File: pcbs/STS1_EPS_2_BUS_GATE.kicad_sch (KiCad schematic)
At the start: 19 parts, among them Q5 SI7135DP-T1-GE3, Q6 2N7002, U13 4082, U3 TPS2420RSAT

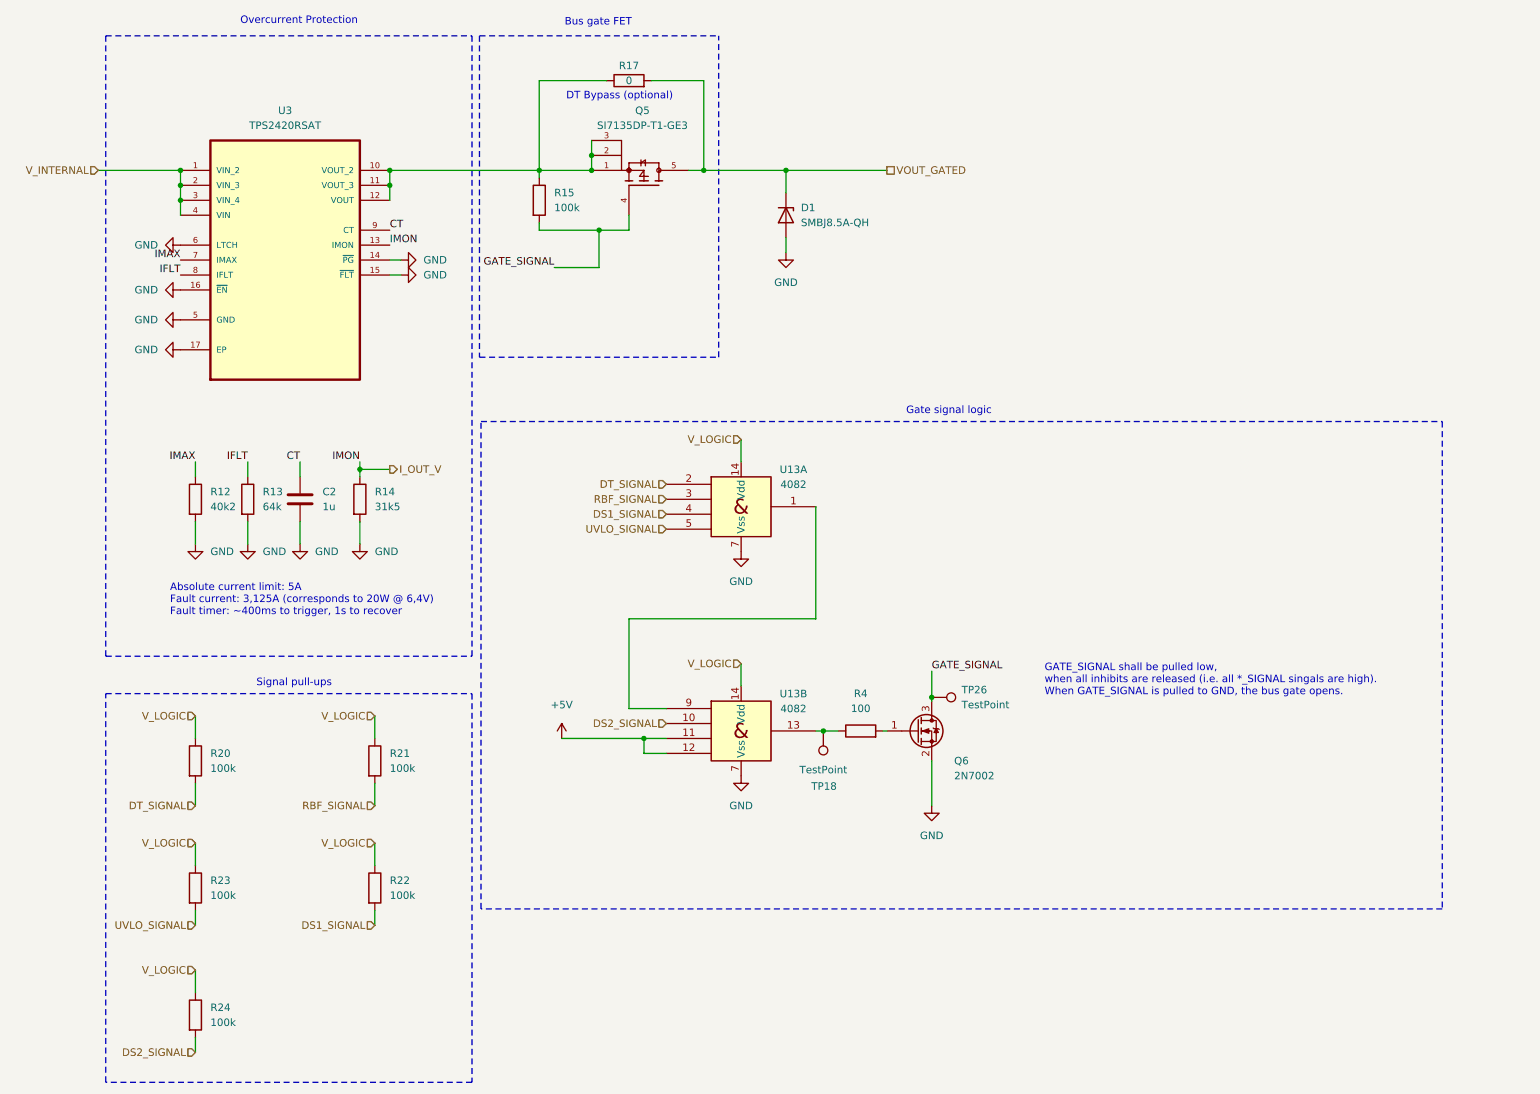
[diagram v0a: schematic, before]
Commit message: Fixed some warnings and errors.
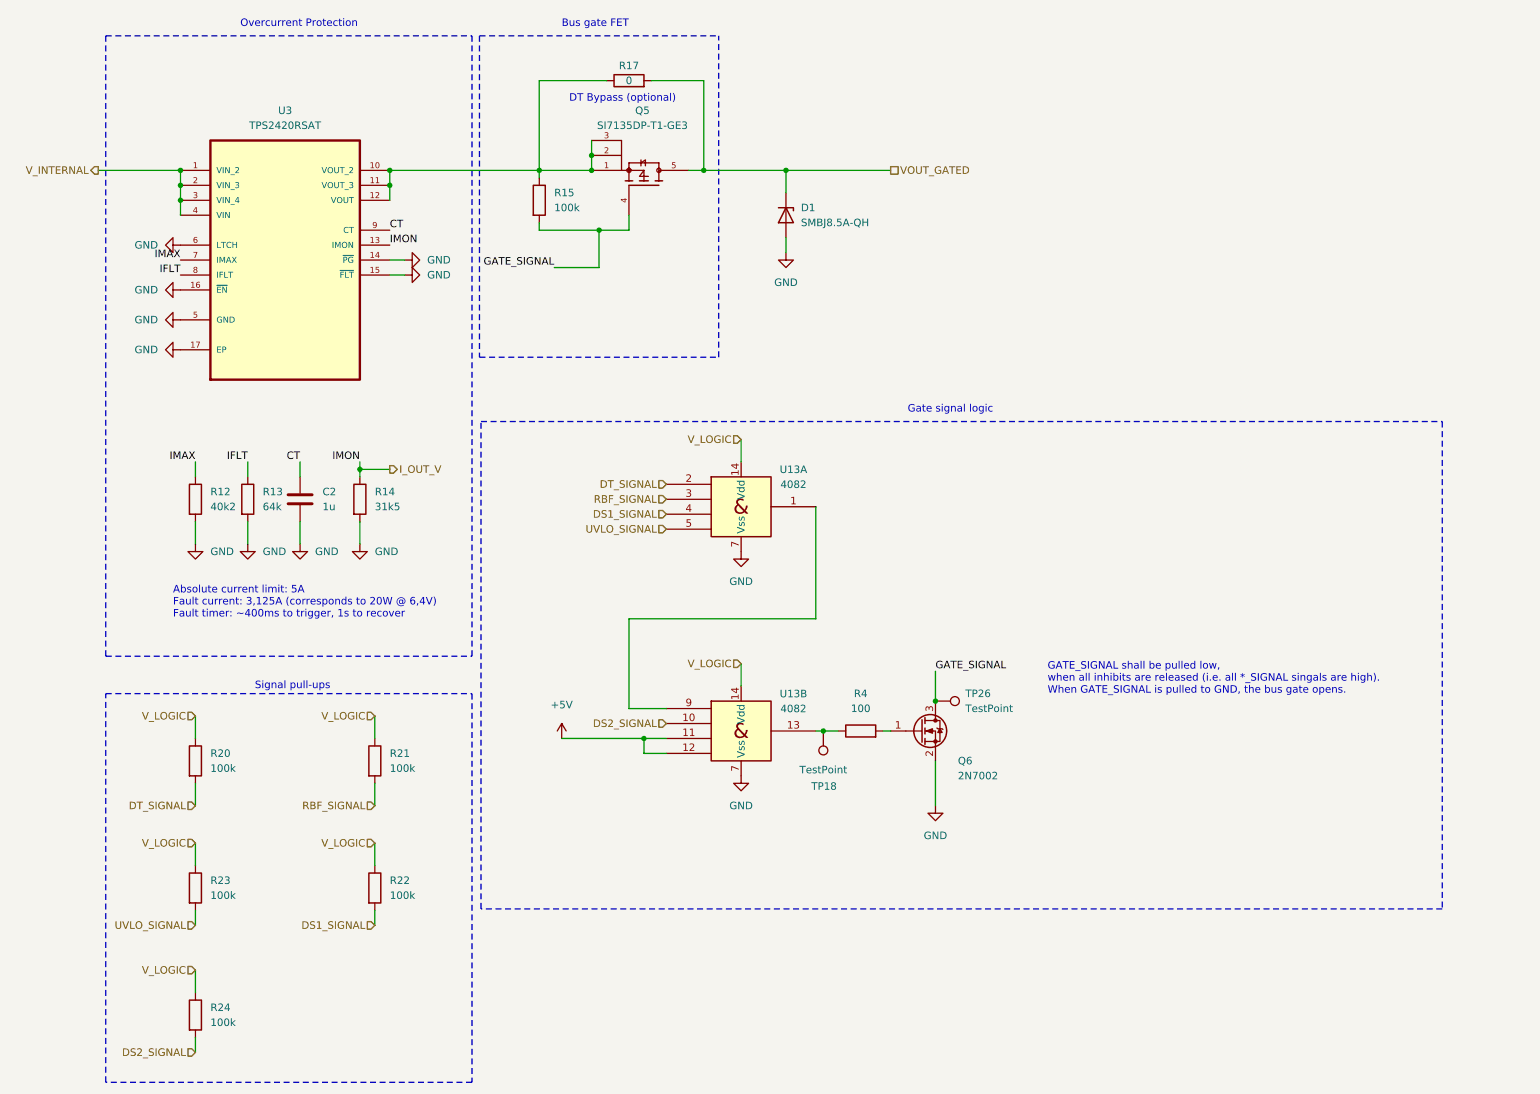
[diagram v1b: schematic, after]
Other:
- moved on the sheet: Q6, TP26
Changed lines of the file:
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@@
 	)
 	(junction
-		(at 168.275 128.905)
+		(at 168.91 129.54)
 		(diameter 0)
 		(color 0 0 0 0)
@@
 	(wire
 		(pts
-			(xy 143.51 39.37) (xy 160.655 39.37)
+			(xy 143.51 39.37) (xy 161.29 39.37)
 		)
 		(stroke
@@
 	(wire
 		(pts
-			(xy 78.105 54.61) (xy 76.2 54.61)
+			(xy 78.74 54.61) (xy 76.2 54.61)
 		)
 		(stroke
@@
 	(wire
 		(pts
-			(xy 160.02 134.62) (xy 160.655 134.62)
+			(xy 160.02 134.62) (xy 161.29 134.62)
 		)
 		(stroke
@@
 	(wire
 		(pts
-			(xy 168.275 124.46) (xy 168.275 128.905)
+			(xy 168.91 124.46) (xy 168.91 129.54)
 		)
 		(stroke
@@
 	(wire
 		(pts
-			(xy 78.105 57.15) (xy 76.2 57.15)
+			(xy 78.74 57.15) (xy 76.2 57.15)
 		)
 		(stroke
@@
 	(wire
 		(pts
-			(xy 168.275 139.7) (xy 168.275 147.32)
+			(xy 168.91 139.7) (xy 168.91 147.32)
 		)
 		(stroke
@@
 	(wire
 		(pts
-			(xy 168.275 128.905) (xy 168.275 129.54)
-		)
-		(stroke
-			(width 0)
-			(type default)
-		)
-	)
-	(wire
-		(pts
 			(xy 129.54 39.37) (xy 143.51 39.37)
 		)
@@
 	(text "Signal pull-ups"
 		(exclude_from_sim no)
-		(at 59.944 126.492 0)
+		(at 59.69 127 0)
 		(effects
 			(font
@@
 	(text "Gate signal logic"
 		(exclude_from_sim no)
-		(at 171.196 80.264 0)
+		(at 171.45 80.01 0)
 		(effects
 			(font
@@
 	(text "Overcurrent Protection\n"
 		(exclude_from_sim no)
-		(at 50.8 14.732 0)
+		(at 50.8 15.24 0)
 		(effects
 			(font
@@
 	(text "Bus gate FET"
 		(exclude_from_sim no)
-		(at 105.918 14.986 0)
+		(at 105.41 15.24 0)
 		(effects
 			(font
@@
 	(text "Absolute current limit: 5A\nFault current: 3,125A (corresponds to 20W @ 6,4V)\nFault timer: ~400ms to trigger, 1s to recover"
 		(exclude_from_sim no)
-		(at 38.862 115.1636 0)
+		(at 39.37 115.57 0)
 		(effects
 			(font
@@
 	(text "DT Bypass (optional)\n"
 		(exclude_from_sim no)
-		(at 106.172 27.5336 0)
+		(at 106.68 27.94 0)
 		(effects
 			(font
@@
 	(text "GATE_SIGNAL shall be pulled low,\nwhen all inhibits are released (i.e. all *_SIGNAL singals are high). \nWhen GATE_SIGNAL is pulled to GND, the bus gate opens."
 		(exclude_from_sim no)
-		(at 187.452 125.984 0)
+		(at 187.96 125.73 0)
 		(effects
 			(font
@@
 	)
 	(label "GATE_SIGNAL"
-		(at 168.275 124.46 0)
+		(at 168.91 124.46 0)
 		(fields_autoplaced yes)
 		(effects
@@
 	(hierarchical_label "VOUT_GATED"
 		(shape passive)
-		(at 160.655 39.37 0)
+		(at 161.29 39.37 0)
 		(fields_autoplaced yes)
 		(effects
@@
 	)
 	(hierarchical_label "V_INTERNAL"
-		(shape input)
+		(shape output)
 		(at 26.67 39.37 180)
 		(fields_autoplaced yes)
@@
 	(symbol
 		(lib_id "power:GND")
-		(at 78.105 54.61 90)
+		(at 78.74 54.61 90)
 		(unit 1)
 		(exclude_from_sim no)
@@
 		(fields_autoplaced yes)
 		(property "Reference" "#PWR044"
-			(at 84.455 54.61 0)
+			(at 85.09 54.61 0)
 			(effects
 				(font
@@
 		)
 		(property "Value" "GND"
-			(at 81.915 54.6099 90)
+			(at 82.55 54.6099 90)
 			(effects
 				(font
@@
 		)
 		(property "Footprint" ""
-			(at 78.105 54.61 0)
+			(at 78.74 54.61 0)
 			(effects
 				(font
@@
 		)
 		(property "Datasheet" ""
-			(at 78.105 54.61 0)
+			(at 78.74 54.61 0)
 			(effects
 				(font
@@
 			)
 		)
-		(property "Description" ""
-			(at 78.105 54.61 0)
+		(property "Description" "Power symbol creates a global label with name \"GND\" , ground"
+			(at 78.74 54.61 0)
 			(effects
 				(font
@@
 	(symbol
 		(lib_id "Transistor_FET:2N7002")
-		(at 165.735 134.62 0)
+		(at 166.37 134.62 0)
 		(unit 1)
 		(exclude_from_sim no)
@@
 		(dnp no)
 		(property "Reference" "Q6"
-			(at 172.085 139.7 0)
+			(at 172.72 139.7 0)
 			(effects
 				(font
@@
 		)
 		(property "Value" "2N7002"
-			(at 172.085 142.24 0)
+			(at 172.72 142.24 0)
 			(effects
 				(font
@@
 		)
 		(property "Footprint" "Package_TO_SOT_SMD:SOT-23"
-			(at 170.815 136.525 0)
+			(at 171.45 136.525 0)
 			(effects
 				(font
@@
 		)
 		(property "Datasheet" "https://www.onsemi.com/pub/Collateral/NDS7002A-D.PDF"
-			(at 165.735 134.62 0)
+			(at 166.37 134.62 0)
 			(effects
 				(font
@@
 			)
 		)
-		(property "Description" ""
-			(at 165.735 134.62 0)
+		(property "Description" "0.115A Id, 60V Vds, N-Channel MOSFET, SOT-23"
+			(at 166.37 134.62 0)
 			(effects
 				(font
@@
 	(symbol
 		(lib_id "Connector:TestPoint")
-		(at 168.275 128.905 270)
+		(at 168.91 129.54 270)
 		(unit 1)
 		(exclude_from_sim no)
@@
 		(fields_autoplaced yes)
 		(property "Reference" "TP26"
-			(at 173.355 127.6349 90)
+			(at 173.99 128.2699 90)
 			(effects
 				(font
@@
 		)
 		(property "Value" "TestPoint"
-			(at 173.355 130.1749 90)
+			(at 173.99 130.8099 90)
 			(effects
 				(font
@@
 		)
 		(property "Footprint" "TestPoint:TestPoint_THTPad_D1.0mm_Drill0.5mm"
-			(at 168.275 133.985 0)
+			(at 168.91 134.62 0)
 			(effects
 				(font
@@
 		)
 		(property "Datasheet" "~"
-			(at 168.275 133.985 0)
+			(at 168.91 134.62 0)
 			(effects
 				(font
@@
 		)
 		(property "Description" ""
-			(at 168.275 128.905 0)
+			(at 168.91 129.54 0)
 			(effects
 				(font
@@
 			)
 		)
-		(property "Description" ""
+		(property "Description" "Power symbol creates a global label with name \"GND\" , ground"
 			(at 143.51 53.34 0)
 			(effects
@@
 			)
 		)
-		(property "Description" ""
+		(property "Description" "Power symbol creates a global label with name \"GND\" , ground"
 			(at 71.12 102.87 0)
 			(effects
@@
 			)
 		)
-		(property "Description" ""
+		(property "Description" "Power symbol creates a global label with name \"+5V\""
 			(at 105.41 135.89 0)
 			(effects
@@
 			)
 		)
-		(property "Description" ""
+		(property "Description" "Power symbol creates a global label with name \"GND\" , ground"
 			(at 40.64 64.77 0)
 			(effects
@@
 			)
 		)
-		(property "Description" ""
+		(property "Description" "Power symbol creates a global label with name \"GND\" , ground"
 			(at 135.89 142.24 0)
 			(effects
@@
 	(symbol
 		(lib_id "power:GND")
-		(at 168.275 147.32 0)
+		(at 168.91 147.32 0)
 		(unit 1)
 		(exclude_from_sim no)
@@
 		(fields_autoplaced yes)
 		(property "Reference" "#PWR0107"
-			(at 168.275 153.67 0)
+			(at 168.91 153.67 0)
 			(effects
 				(font
@@
 		)
 		(property "Value" "GND"
-			(at 168.275 152.4 0)
+			(at 168.91 152.4 0)
 			(effects
 				(font
@@
 		)
 		(property "Footprint" ""
-			(at 168.275 147.32 0)
+			(at 168.91 147.32 0)
 			(effects
 				(font
@@
 		)
 		(property "Datasheet" ""
-			(at 168.275 147.32 0)
+			(at 168.91 147.32 0)
 			(effects
 				(font
@@
 			)
 		)
-		(property "Description" ""
-			(at 168.275 147.32 0)
+		(property "Description" "Power symbol creates a global label with name \"GND\" , ground"
+			(at 168.91 147.32 0)
 			(effects
 				(font
@@
 			)
 		)
-		(property "Description" ""
+		(property "Description" "Power symbol creates a global label with name \"GND\" , ground"
 			(at 135.89 104.14 0)
 			(effects
@@
 			)
 		)
-		(property "Description" ""
+		(property "Description" "Power symbol creates a global label with name \"GND\" , ground"
 			(at 43.18 102.87 0)
 			(effects
@@
 			)
 		)
-		(property "Description" ""
+		(property "Description" "Power symbol creates a global label with name \"GND\" , ground"
 			(at 60.96 102.87 0)
 			(effects
@@
 	(symbol
 		(lib_id "power:GND")
-		(at 78.105 57.15 90)
+		(at 78.74 57.15 90)
 		(unit 1)
 		(exclude_from_sim no)
@@
 		(fields_autoplaced yes)
 		(property "Reference" "#PWR045"
-			(at 84.455 57.15 0)
+			(at 85.09 57.15 0)
 			(effects
 				(font
@@
 		)
 		(property "Value" "GND"
-			(at 81.915 57.1499 90)
+			(at 82.55 57.1499 90)
 			(effects
 				(font
@@
 		)
 		(property "Footprint" ""
-			(at 78.105 57.15 0)
+			(at 78.74 57.15 0)
 			(effects
 				(font
@@
 		)
 		(property "Datasheet" ""
-			(at 78.105 57.15 0)
+			(at 78.74 57.15 0)
 			(effects
 				(font
@@
 			)
 		)
-		(property "Description" ""
-			(at 78.105 57.15 0)
+		(property "Description" "Power symbol creates a global label with name \"GND\" , ground"
+			(at 78.74 57.15 0)
 			(effects
 				(font
@@
 			)
 		)
-		(property "Description" ""
+		(property "Description" "Power symbol creates a global label with name \"GND\" , ground"
 			(at 40.64 52.07 0)
 			(effects
@@
 			)
 		)
-		(property "Description" ""
+		(property "Description" "Power symbol creates a global label with name \"GND\" , ground"
 			(at 40.64 59.69 0)
 			(effects
@@
 			)
 		)
-		(property "Description" ""
+		(property "Description" "Power symbol creates a global label with name \"GND\" , ground"
 			(at 52.07 102.87 0)
 			(effects
@@
 			)
 		)
-		(property "Description" ""
+		(property "Description" "Power symbol creates a global label with name \"GND\" , ground"
 			(at 40.64 69.85 0)
 			(effects
